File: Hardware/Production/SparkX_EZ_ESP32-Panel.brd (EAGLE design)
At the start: 198.4 x 96 mm, 2406 parts, among them Q1 MBT3904DW1T1, Q10 MBT3904DW1T1, Q11 MBT3904DW1T1, Q12 MBT3904DW1T1, Q13 MBT3904DW1T1, Q14 MBT3904DW1T1, Q15 MBT3904DW1T1, Q16 MBT3904DW1T1, Q17 MBT3904DW1T1, Q18 MBT3904DW1T1, Q19 MBT3904DW1T1, Q2 MBT3904DW1T1, Q20 MBT3904DW1T1, Q21 MBT3904DW1T1, Q22 MBT3904DW1T1, Q23 MBT3904DW1T1, Q24 MBT3904DW1T1, Q25 MBT3904DW1T1, Q26 MBT3904DW1T1, Q27 MBT3904DW1T1, Q28 MBT3904DW1T1, Q29 MBT3904DW1T1, Q3 MBT3904DW1T1, Q30 MBT3904DW1T1, Q31 MBT3904DW1T1, Q32 MBT3904DW1T1, Q4 MBT3904DW1T1, Q5 MBT3904DW1T1, Q6 MBT3904DW1T1, Q7 MBT3904DW1T1, Q8 MBT3904DW1T1, Q9 MBT3904DW1T1, U1 MIC5219 3.3V, U10 W25QXX128MBIT-6X5-SKINNY_CENT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, U100 MIC5219 3.3V, U101 ESP32, U102 W25QXX128MBIT-6X5-SKINNY_CENT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, U103 CP2102N, U104 MIC5219 3.3V, U105 ESP32, U106 W25QXX128MBIT-6X5-SKINNY_CENT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, U107 CP2102N, U108 MIC5219 3.3V, U109 ESP32, U11 CP2102N, U110 W25QXX128MBIT-6X5-SKINNY_CENT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, U111 CP2102N, U112 MIC5219 3.3V, U113 ESP32, U114 W25QXX128MBIT-6X5-SKINNY_CENT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, U115 CP2102N, U116 MIC5219 3.3V, U117 ESP32, U118 W25QXX128MBIT-6X5-SKINNY_CENT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, U119 CP2102N, U12 MIC5219 3.3V, U120 MIC5219 3.3V, U121 ESP32, U122 W25QXX128MBIT-6X5-SKINNY_CENT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, U123 CP2102N, U124 MIC5219 3.3V, U125 ESP32, U126 W25QXX128MBIT-6X5-SKINNY_CENT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, U127 CP2102N, U128 MIC5219 3.3V, U13 ESP32, U14 W25QXX128MBIT-6X5-SKINNY_CENT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, U15 CP2102N, U16 MIC5219 3.3V, U17 ESP32, U18 W25QXX128MBIT-6X5-SKINNY_CENT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, U19 CP2102N, U2 ESP32, U20 MIC5219 3.3V, U21 ESP32, U22 W25QXX128MBIT-6X5-SKINNY_CENT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, U23 CP2102N, U24 MIC5219 3.3V, U25 ESP32, U26 W25QXX128MBIT-6X5-SKINNY_CENT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

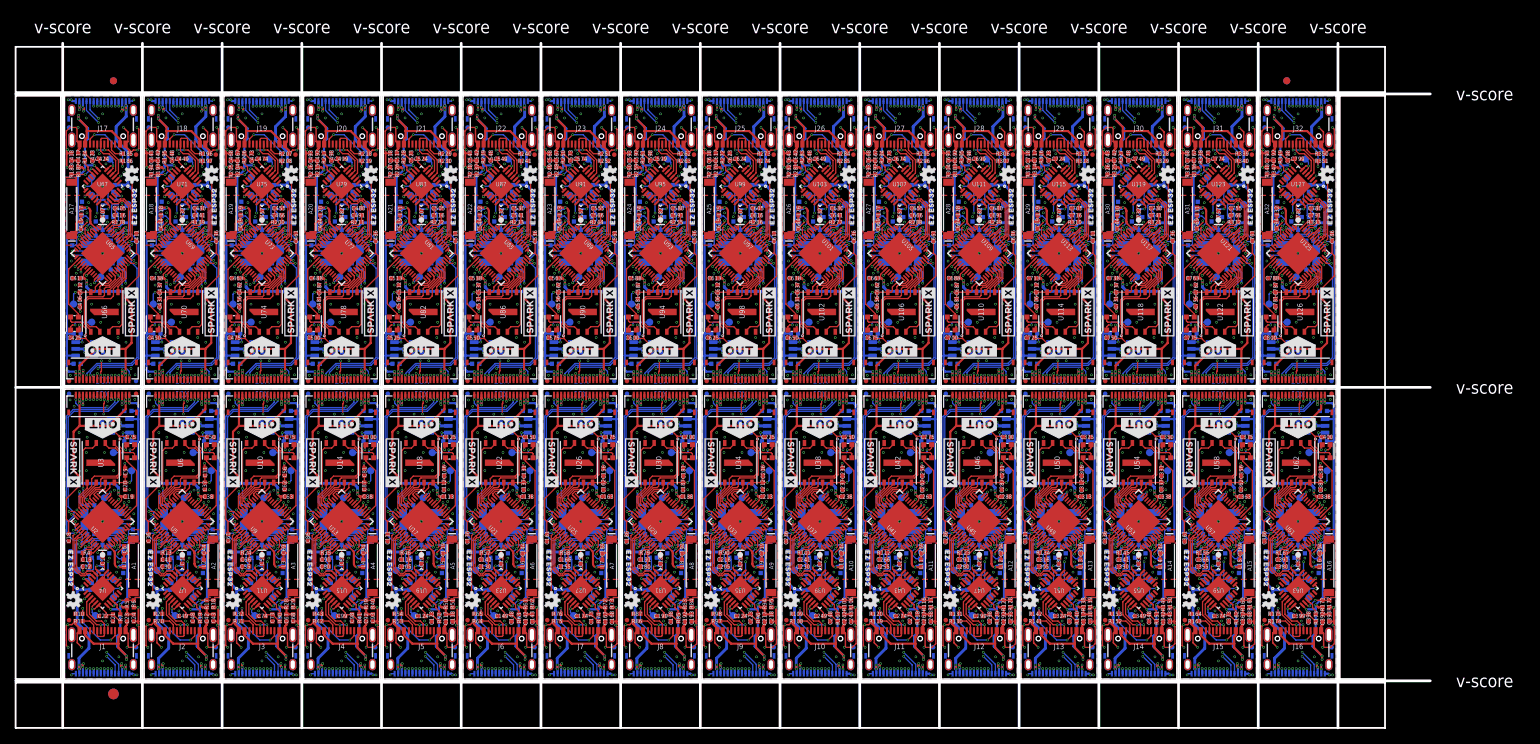
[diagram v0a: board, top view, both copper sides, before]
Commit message: Updates for JLCPCB manufacture
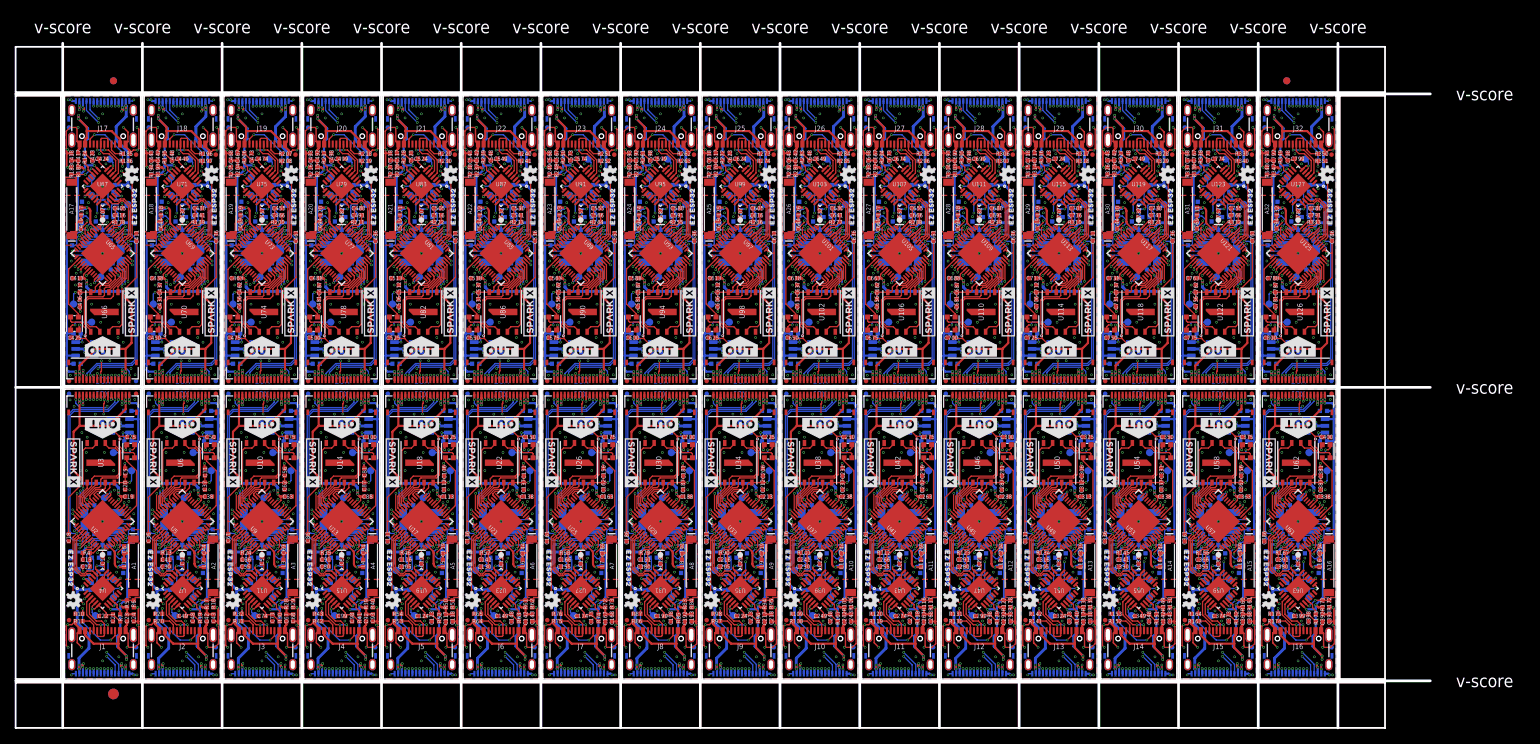
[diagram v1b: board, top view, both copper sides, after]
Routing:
- net CS39: track 43.0 -> 45.3 mm
- net CS93: track 43.0 -> 45.3 mm
- net CS9: track 43.0 -> 45.3 mm
- net CS6: track 43.0 -> 45.3 mm
- net CS42: track 43.0 -> 45.3 mm
- net CS36: track 43.0 -> 45.3 mm
- net CS27: track 43.0 -> 45.3 mm
- net CS24: track 43.0 -> 45.3 mm
- net CS84: track 43.0 -> 45.3 mm
- net CS78: track 43.0 -> 45.3 mm
- net CS48: track 43.0 -> 45.3 mm
- net CS30: track 43.0 -> 45.3 mm
- net CS3: track 43.0 -> 45.3 mm
- net CS0: track 43.0 -> 45.3 mm
- net CS90: track 43.0 -> 45.3 mm
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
